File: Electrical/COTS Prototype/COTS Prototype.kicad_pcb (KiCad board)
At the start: 2 copper layers, 100 x 80 mm, 20 parts, among them J3 Raspberry_Pi_2_3, U1 MCP73831-2-OT, U2 TPS61090

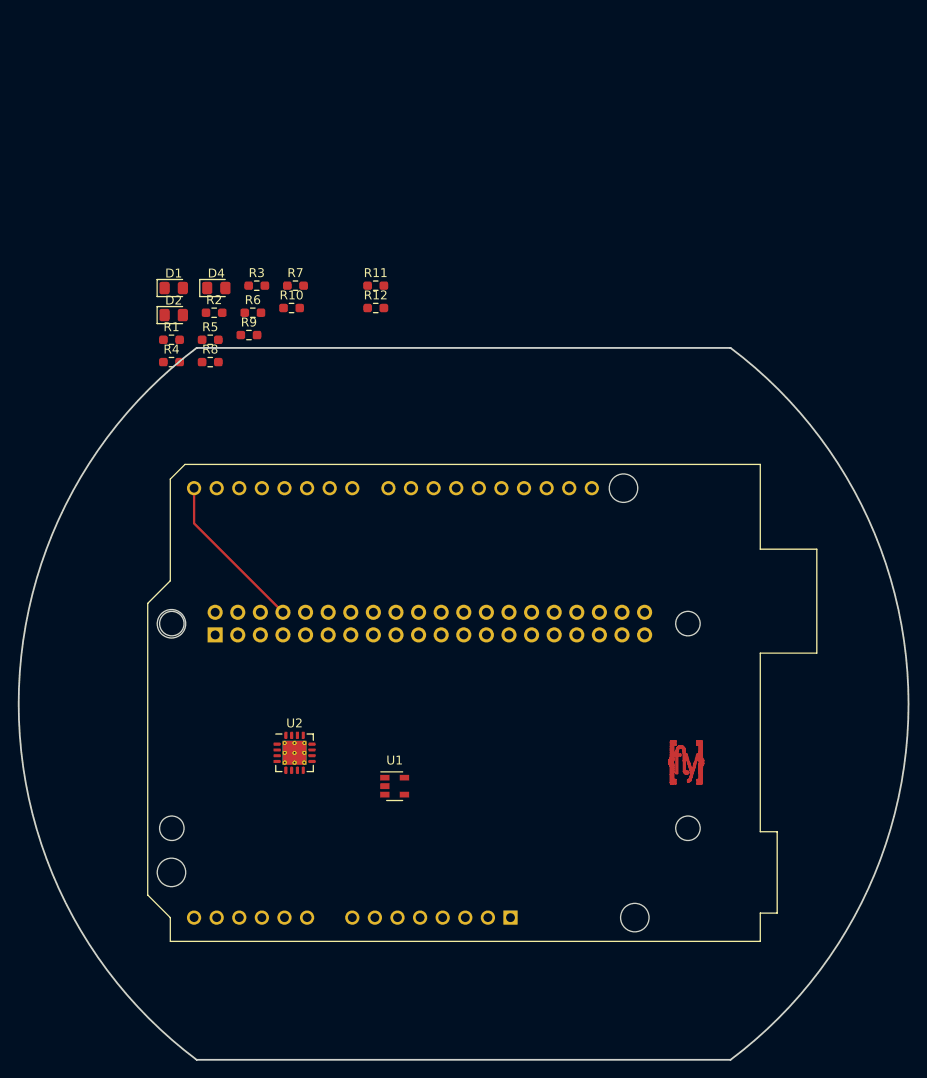
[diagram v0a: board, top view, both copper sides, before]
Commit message: working on schematics
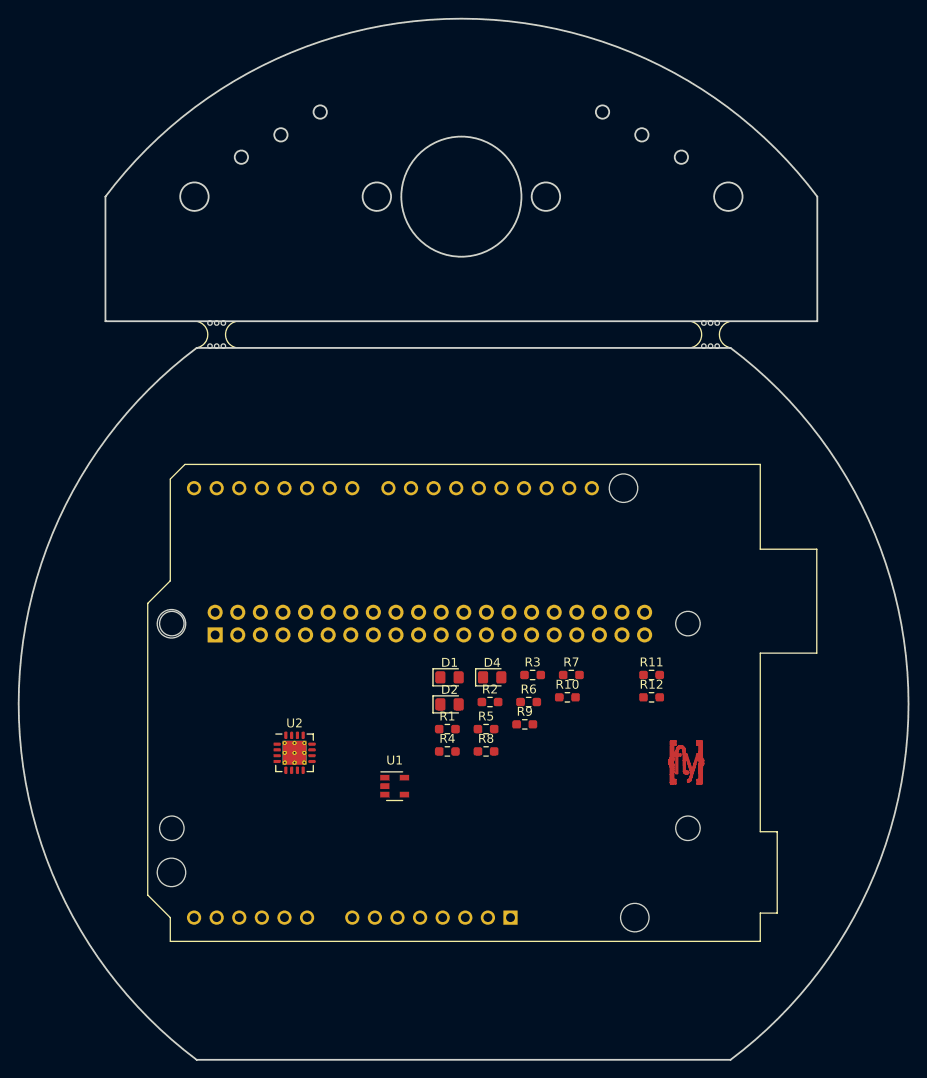
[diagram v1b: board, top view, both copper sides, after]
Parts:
- added mouse-bite-3mm-slot: VAL**, Panelization:mouse-bite-3mm-slot, F.Cu at (231.0, 78.2)
- added mouse-bite-3mm-slot: VAL**, Panelization:mouse-bite-3mm-slot, F.Cu at (175.5, 78.2)
- moved D1 53.6 mm to (201.7, 116.8)
- moved D2 53.6 mm to (201.7, 119.8)
- moved D4 53.6 mm to (206.5, 116.8)
- moved R1 53.6 mm to (201.4, 122.6)
- moved R10 53.6 mm to (214.9, 119.0)
- moved R11 53.6 mm to (224.4, 116.5)
- moved R12 53.6 mm to (224.4, 119.0)
- moved R2 53.6 mm to (206.2, 119.5)
- moved R3 53.6 mm to (211.0, 116.5)
- moved R4 53.6 mm to (201.4, 125.1)
- moved R5 53.6 mm to (205.8, 122.6)
- moved R6 53.6 mm to (210.6, 119.5)
- moved R7 53.6 mm to (215.4, 116.5)
- moved R8 53.6 mm to (205.8, 125.1)
- moved R9 53.6 mm to (210.1, 122.1)
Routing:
- net RPi_to_uC: track 18.1 -> 0.00 mm
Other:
- board size 100 x 80 mm -> 100 x 117 mm
